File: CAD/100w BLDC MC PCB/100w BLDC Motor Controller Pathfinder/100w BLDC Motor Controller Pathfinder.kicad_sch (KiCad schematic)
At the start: 23 parts, among them SW1 PTS815 SJM 250 SMTR LFS, U1 RP2040, U2 W25Q128JVS, Y1 ABLS-12.000MHZ-B4-T

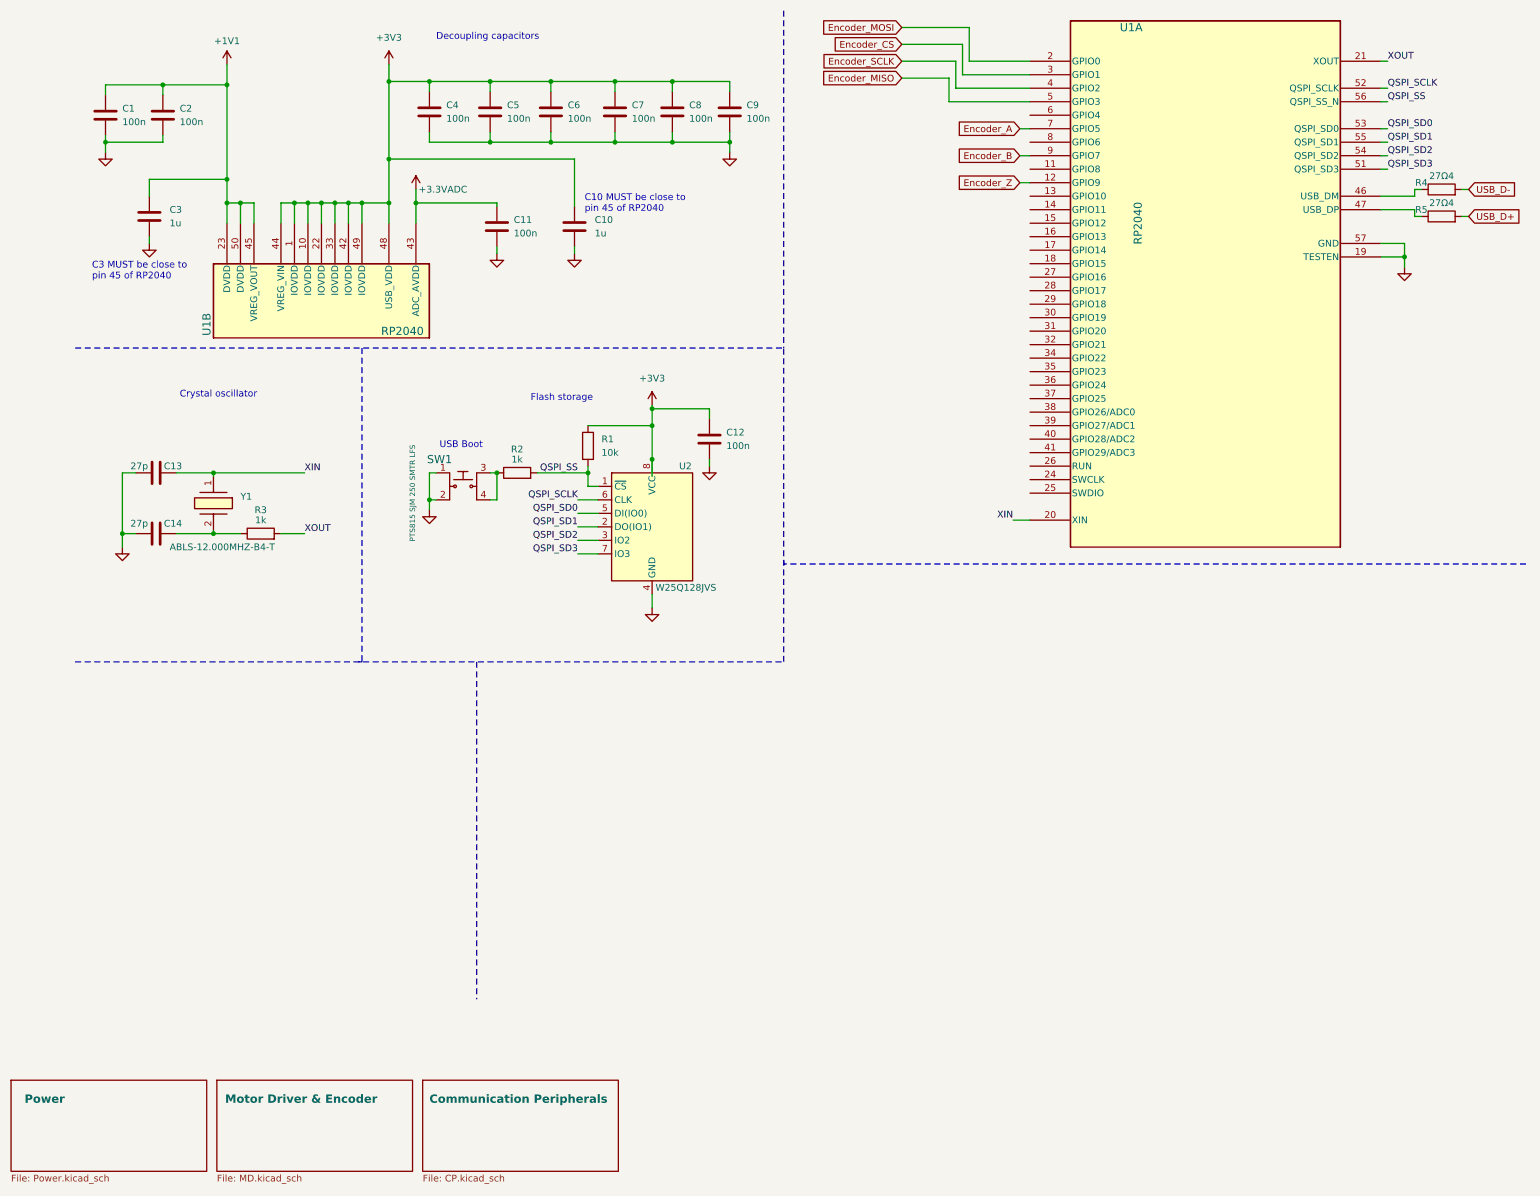
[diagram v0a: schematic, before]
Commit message: Errores pero que probablemente no son errores
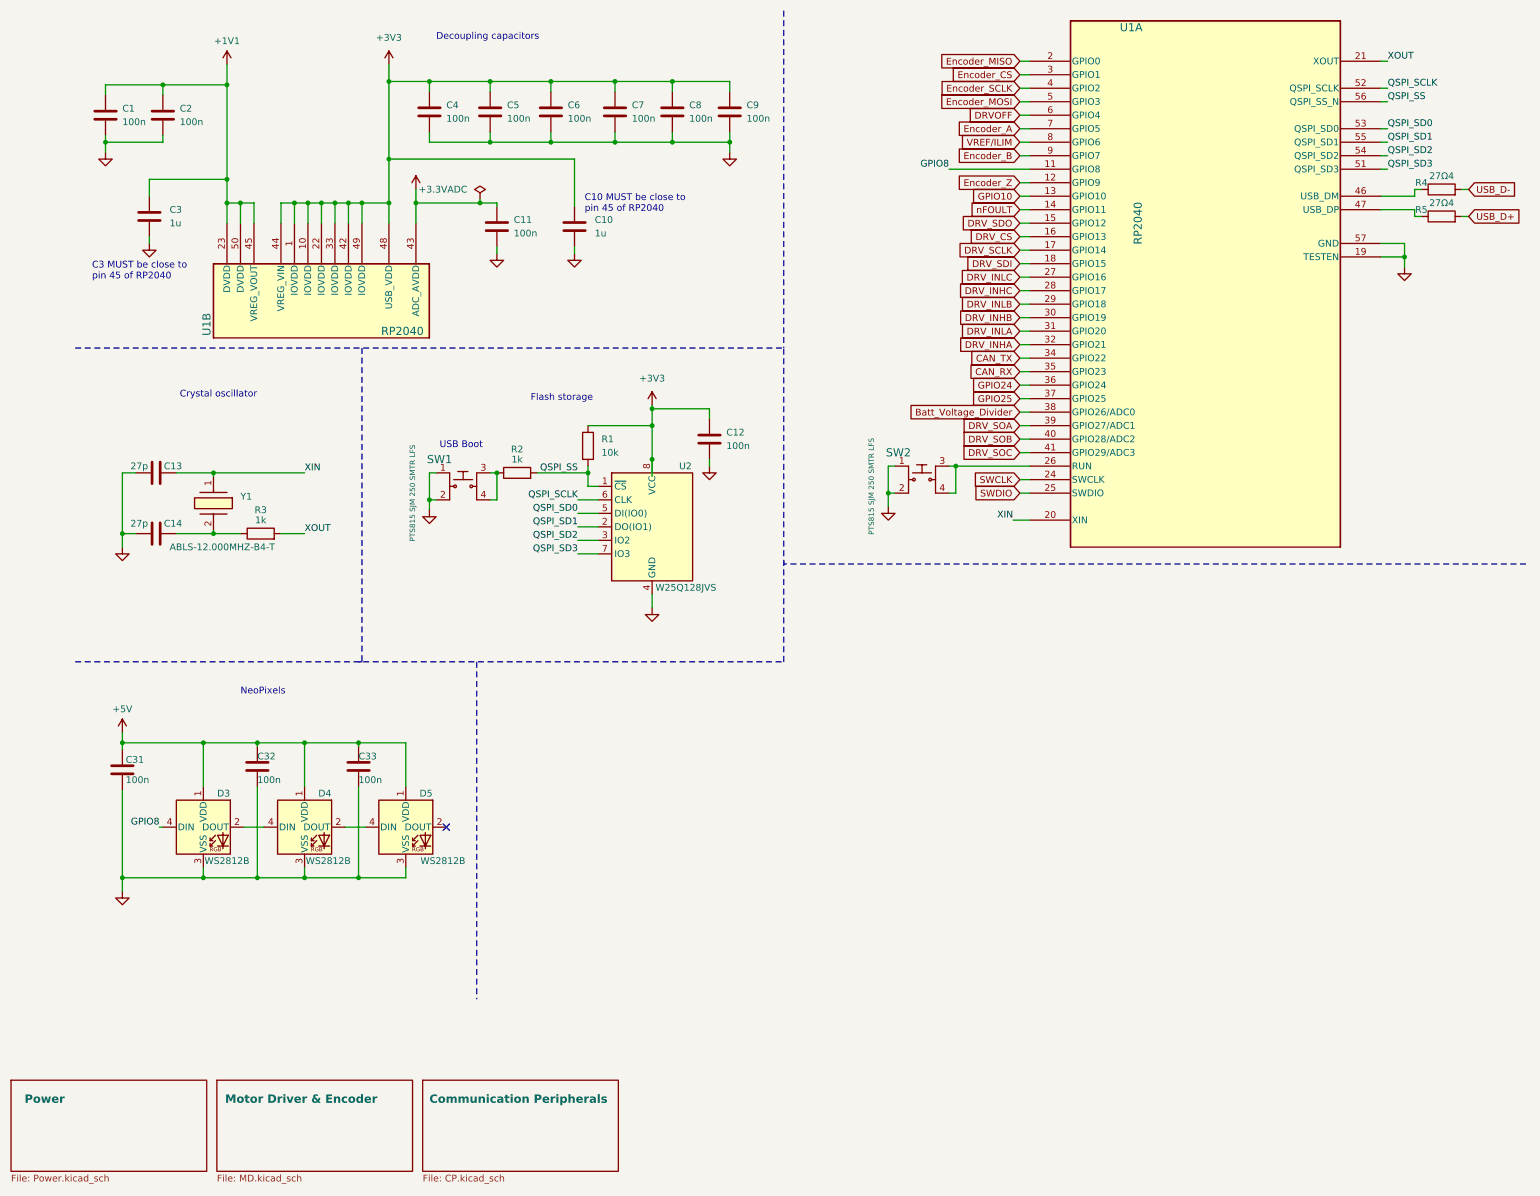
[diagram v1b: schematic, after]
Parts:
- added C31, C32, C33: 100n, symbol Device:C
- added D3, D4, D5: WS2812B, LED_SMD:LED_WS2812B_PLCC4_5.0x5.0mm_P3.2mm, symbol LED:WS2812B
- added SW2: PTS815 SJM 250 SMTR LFS, SW4_PTS815 SJM 250 SMTR LFS_CNK, symbol 2024-01-22_02-04-17:PTS815_SJM_250_SMTR_LFS
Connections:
- net Encoder_MISO: now also U1.2 (GPIO0); no longer U1.5 (GPIO3)
- net Encoder_MOSI: now also U1.5 (GPIO3); no longer U1.2 (GPIO0)
- net GND: now also C31.2, C32.2, C33.2, D3.3 (VSS), D4.3 (VSS), D5.3 (VSS), SW2.1, SW2.2
- net GPIO8: now reaches U1.11 (GPIO8)
- net GPIO8: now also D3.4 (DIN)
- net GPIO10: now reaches U1.13 (GPIO10)
- net nFOULT: now reaches U1.14 (GPIO11)
- net DRV_SDO: now reaches U1.15 (GPIO12)
- net DRV_CS: now reaches U1.16 (GPIO13)
- net DRV_SCLK: now reaches U1.17 (GPIO14)
- net DRV_SDI: now reaches U1.18 (GPIO15)
- net SWCLK: now reaches U1.24 (SWCLK)
- net SWDIO: now reaches U1.25 (SWDIO)
- net at U1.26 (RUN): now also SW2.3, SW2.4
- net DRV_INLC: now reaches U1.27 (GPIO16)
- net DRV_INHC: now reaches U1.28 (GPIO17)
- net DRV_INLB: now reaches U1.29 (GPIO18)
- net DRV_INHB: now reaches U1.30 (GPIO19)
- net DRV_INLA: now reaches U1.31 (GPIO20)
- net DRV_INHA: now reaches U1.32 (GPIO21)
- net CAN_TX: now reaches U1.34 (GPIO22)
- net CAN_RX: now reaches U1.35 (GPIO23)
- net GPIO24: now reaches U1.36 (GPIO24)
- net GPIO25: now reaches U1.37 (GPIO25)
- net Batt_Voltage_Divider: now reaches U1.38 (GPIO26/ADC0)
- net DRV_SOA: now reaches U1.39 (GPIO27/ADC1)
- net DRV_SOB: now reaches U1.40 (GPIO28/ADC2)
- net DRV_SOC: now reaches U1.41 (GPIO29/ADC3)
- net DRVOFF: now reaches U1.6 (GPIO4)
- net VREF/ILIM: now reaches U1.8 (GPIO6)
- new net: D3.2 (DOUT), D4.4 (DIN)
- new net: D4.2 (DOUT), D5.4 (DIN)
- new net +5V: C31.1, C32.1, C33.1, D3.1 (VDD), D4.1 (VDD), D5.1 (VDD)
- no-connect marks 0 -> 1
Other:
- note added: "NeoPixels"
